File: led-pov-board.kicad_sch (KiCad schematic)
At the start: 18 parts, among them SW1 SW_Push, U1 ATtiny24A-SS

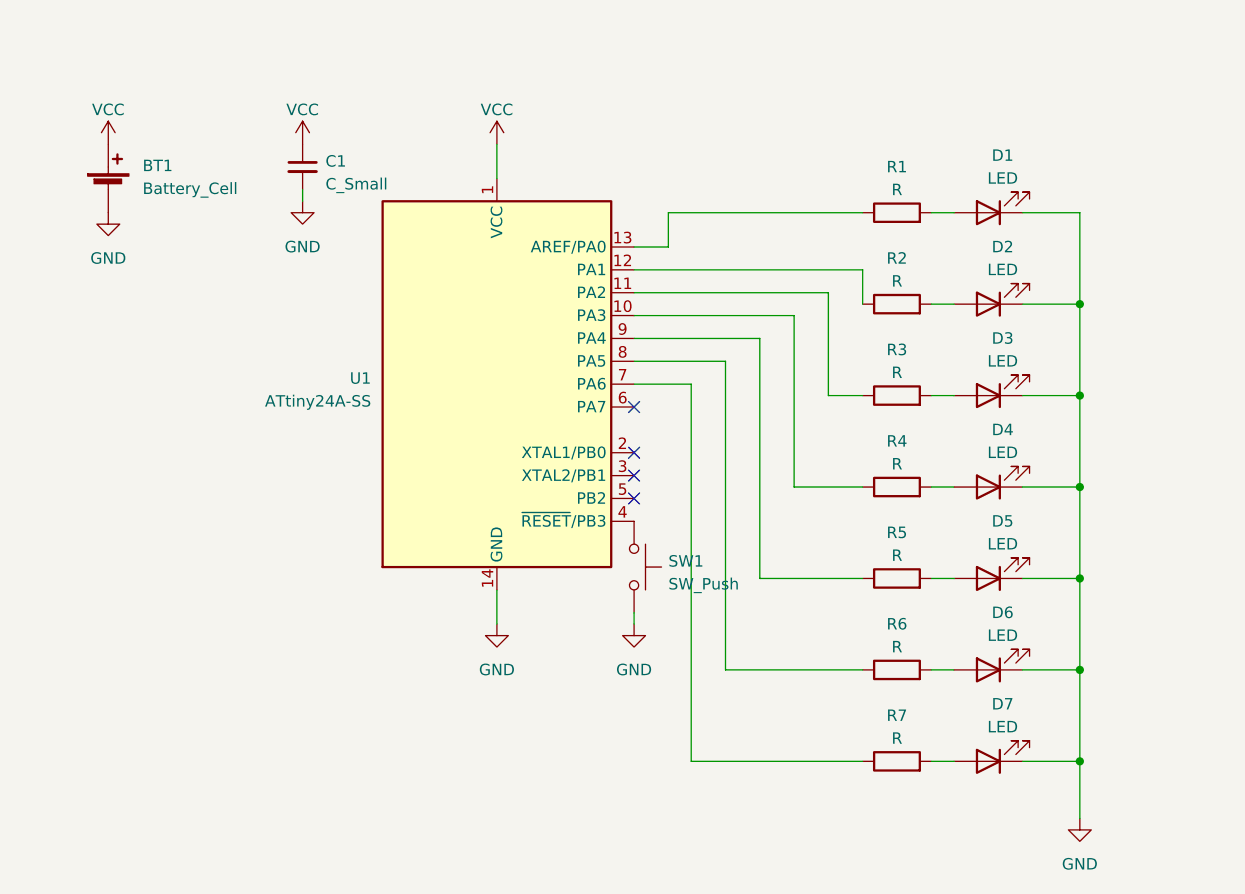
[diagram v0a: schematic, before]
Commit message: add details to schematic
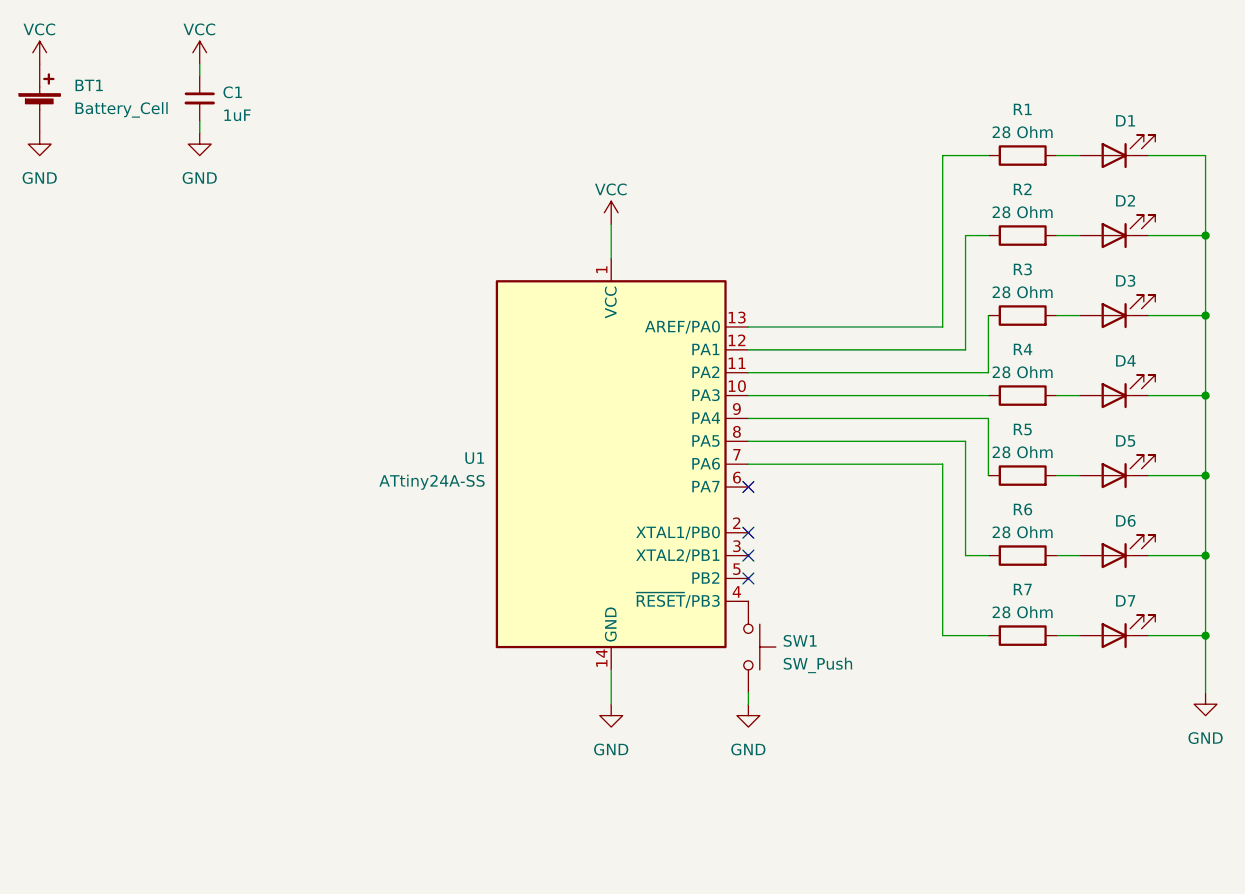
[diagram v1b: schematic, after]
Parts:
- C1: value C_Small -> 1uF
- R1, R2, R3, R4, R5, R6, R7: value R -> 28 Ohm
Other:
- moved on the sheet: BT1, C1, D1, D2, D3, D4, D5, D6, D7, R1, R2, R3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
